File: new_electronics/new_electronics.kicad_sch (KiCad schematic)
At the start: 31 parts, among them M1 Motor_Servo, M2 Motor_Servo, M3 Motor_Servo, M4 Motor_Servo, P1 Pump Aft, P2 Pump Fwd, SW1 Power Switch, SW1 Pump Aft (P5), SW2 Manual/Auto Switch, SW2 Pump Fwd (P4), SW3 SW_SPDT, SW3 Vent Button, SW4 Blow Button, SW4 SW_SPDT, U1 adafruit_metro_mini, U2 buck_converter, U3 MPU-6050

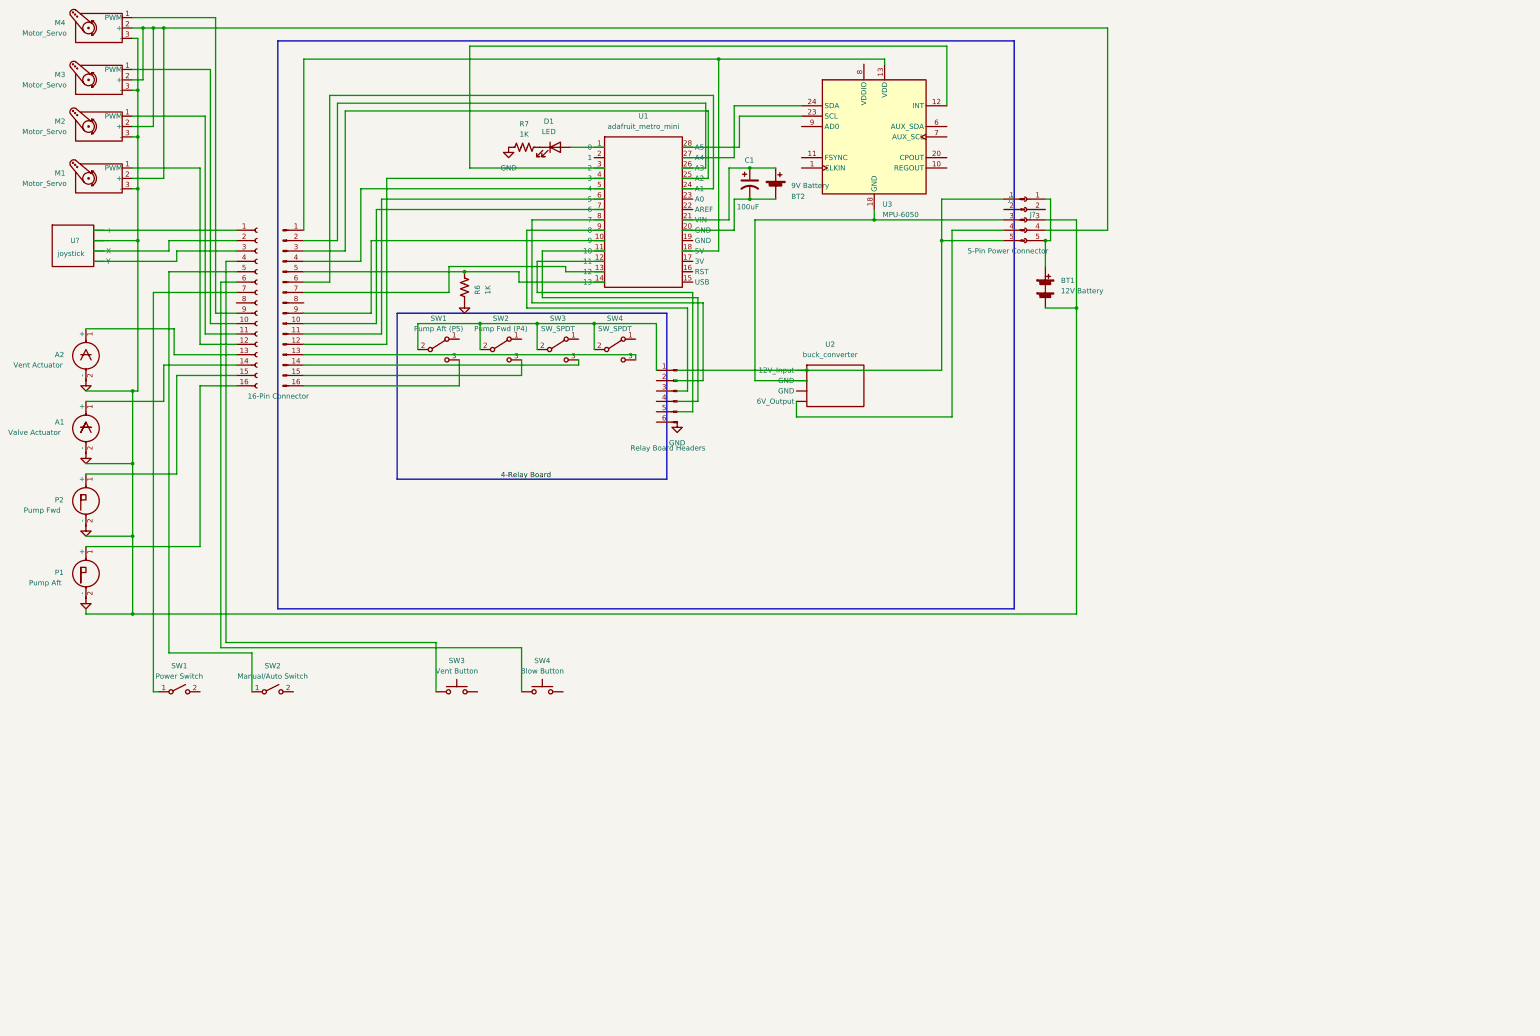
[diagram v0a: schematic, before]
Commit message: 'complete' old schematic and work on new one
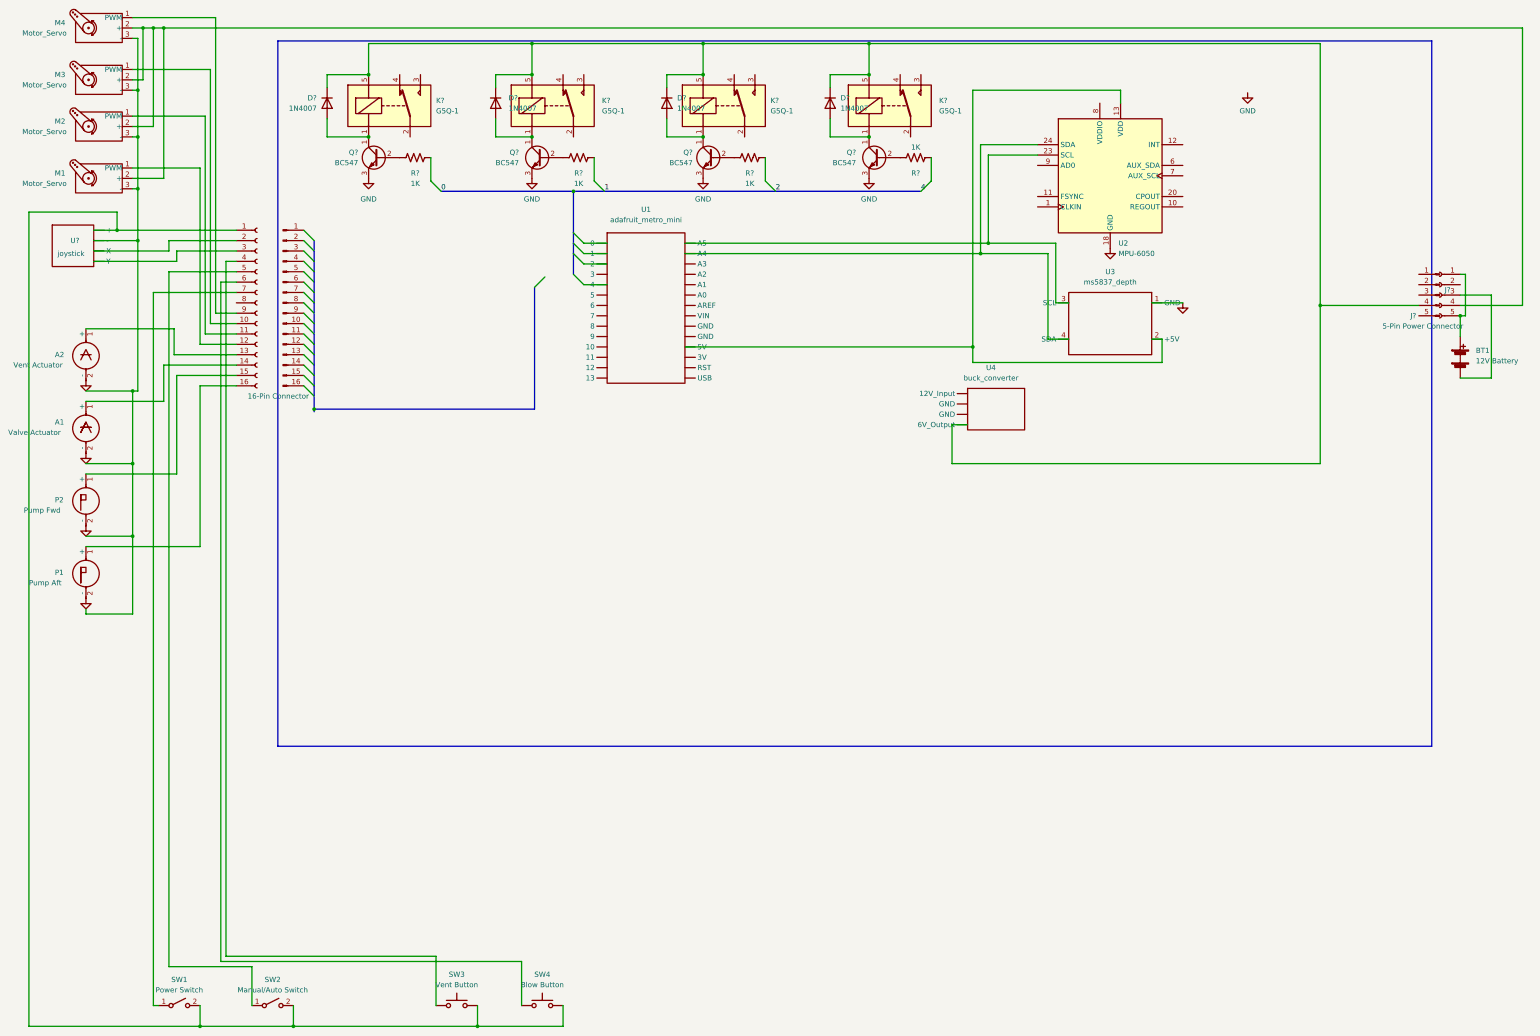
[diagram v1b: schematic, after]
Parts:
- removed BT2: 9V Battery, symbol Device:Battery_Cell
- removed C1: 100uF, symbol Device:C_Polarized_US
- removed D1: LED, symbol Device:LED
- removed J?: Relay Board Headers, symbol Connector:Conn_01x06_Male
- removed R6, R7: 1K, symbol Device:R_US
- removed SW1: Pump Aft (P5), symbol Switch:SW_SPDT
- removed SW2: Pump Fwd (P4), symbol Switch:SW_SPDT
- removed SW3, SW4: SW_SPDT, symbol Switch:SW_SPDT
- removed U2: buck_converter, symbol custom_parts:buck_converter
- removed U3: MPU-6050, Sensor_Motion:InvenSense_QFN-24_4x4mm_P0.5mm, symbol Sensor_Motion:MPU-6050
- added D? (x4): 1N4007, symbol Device:D
- added K? (x4): G5Q-1, Relay_THT:Relay_SPDT_Omron-G5Q-1, symbol Relay:G5Q-1
- added Q? (x4): BC547, Package_TO_SOT_THT:TO-92_Inline, symbol Transistor_BJT:BC547
- added R? (x4): 1K, symbol Device:R_US
- added U2: MPU-6050, Sensor_Motion:InvenSense_QFN-24_4x4mm_P0.5mm, symbol Sensor_Motion:MPU-6050
- added U3: ms5837_depth, symbol custom_parts:ms5837_depth
- added U4: buck_converter, symbol custom_parts:buck_converter
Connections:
- net GND: now also Q?.3 (E), Q?.3 (E), Q?.3 (E), Q?.3 (E), U2.18 (GND), U3.1 (GND)
- net at U1.18 (5V): now also U2.13 (VDD), U3.2 (+5V); no longer J?.1 (Pin_1)
- net at U1.28 (A5): now also U2.23 (SCL), U3.3 (SCL)
- net at U1.27 (A4): now also U2.24 (SDA), U3.4 (SDA)
- net at J?.9 (Pin_9): no longer U1.10 (9)
- net at J?.7 (Pin_7): no longer U1.13 (12)
- net at J?.5 (Pin_5): no longer U1.14 (13)
- net at J?.6 (Pin_6): no longer U1.24 (A1)
- net at J?.3 (Pin_3): no longer U1.25 (A2)
- net at J?.2 (Pin_2): no longer U1.26 (A3)
- net at J?.12 (Pin_12): no longer U1.4 (3)
- net at J?.4 (Pin_4): no longer U1.5 (4)
- net at J?.11 (Pin_11): no longer U1.6 (5)
- net at J?.10 (Pin_10): no longer U1.7 (6)
- net at M1.3 (-), M2.3 (-), M3.3 (-)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: no longer BT1.2 (-), J?.3 (Pin_3)
- net at SW1.2 (B): now also J?.1 (Pin_1), SW2.2 (B), SW3.2, SW4.2, U?. (Y)
- net at U?. (Y): now also J?.3 (Pin_3); no longer J?.1 (Pin_1)
- net at J?.1 (Pin_1): no longer J?.5 (Pin_5)
- net at J?.4 (Pin_4): now also D?.1 (K), D?.1 (K), D?.1 (K), D?.1 (K), K?.5, K?.5, K?.5, K?.5, U4. (GND)
- new net: Q?.2 (B), R?.1 (x4)
- new net: D?.2 (A), K?.1, Q?.1 (C) (x4)
- new net: BT1.2 (-), J?.3 (Pin_3)
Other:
- moved on the sheet: BT1, J?, SW1, SW2, SW3, SW4
